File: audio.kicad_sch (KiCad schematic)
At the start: 31 parts, among them IC4 ES9218PQ, J4 SJ2-35954B-SMT-TR, Y1 ECS-2520SMV-500-GP-TR

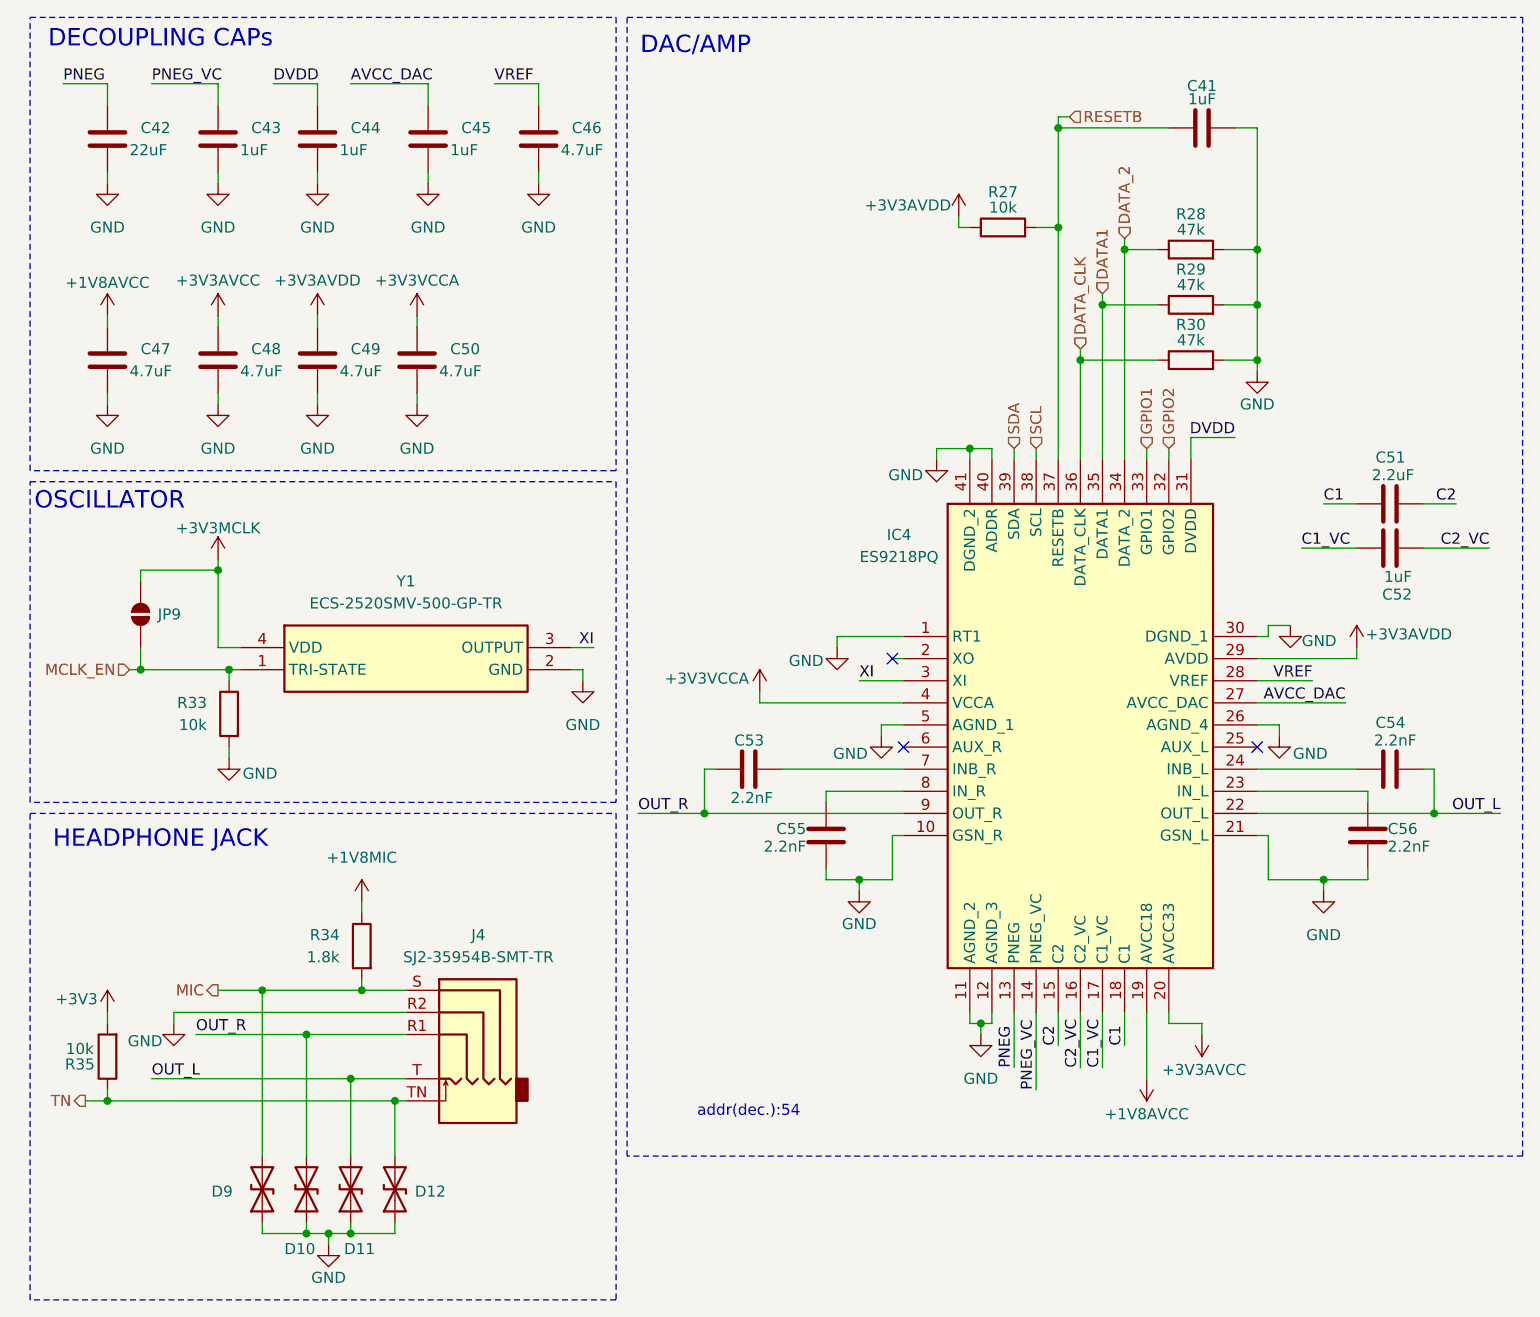
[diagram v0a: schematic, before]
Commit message: layout
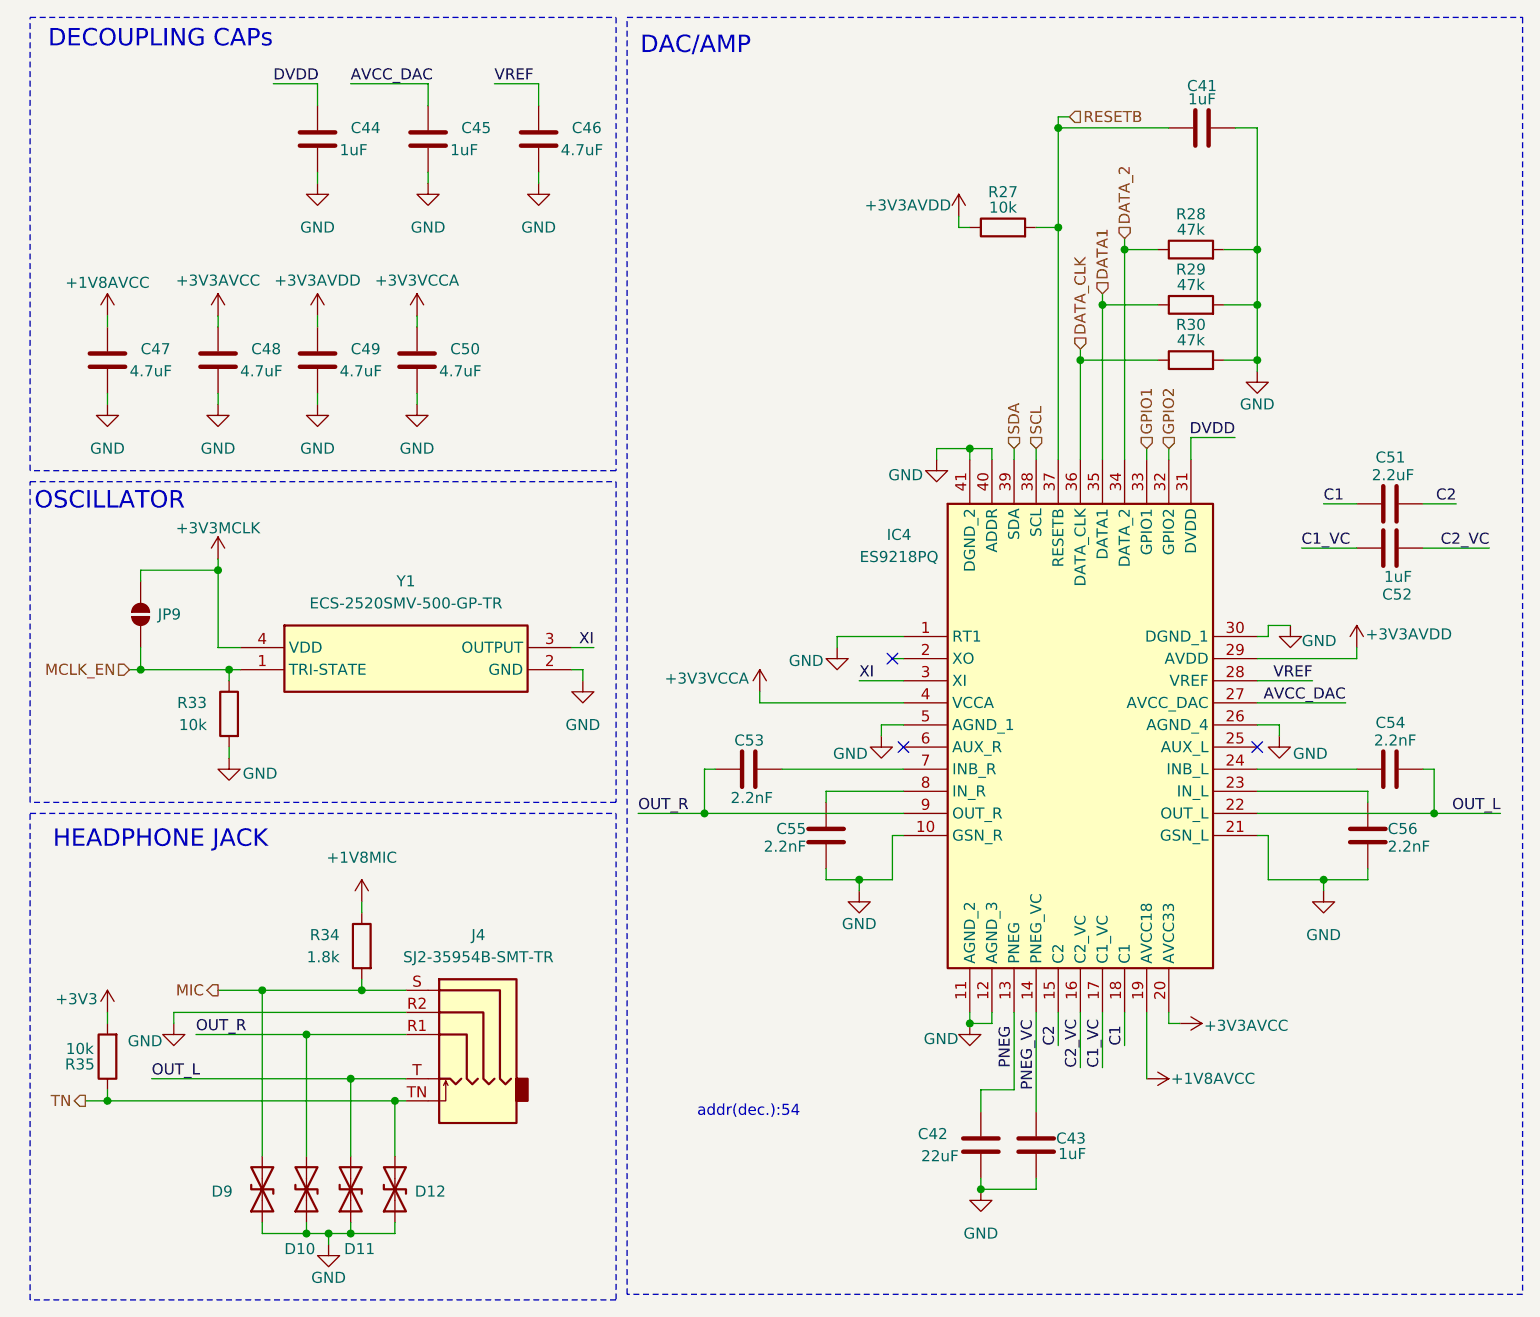
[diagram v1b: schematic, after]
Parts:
- C42: footprint Capacitor_SMD:C_0402_1005Metric -> Capacitor_SMD:C_0603_1608Metric
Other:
- moved on the sheet: C42, C43
